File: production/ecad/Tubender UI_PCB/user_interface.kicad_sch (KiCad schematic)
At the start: 20 parts, among them IC3 SN74LVC1G29DCTR, J1 640387-5, J2 1-640387-0, J3 104031-0811, J4 640387-5, J5 4-1734592-0, J6 4-1734592-0, U5 74HC595, U6 PEC11R-4215K-S0024

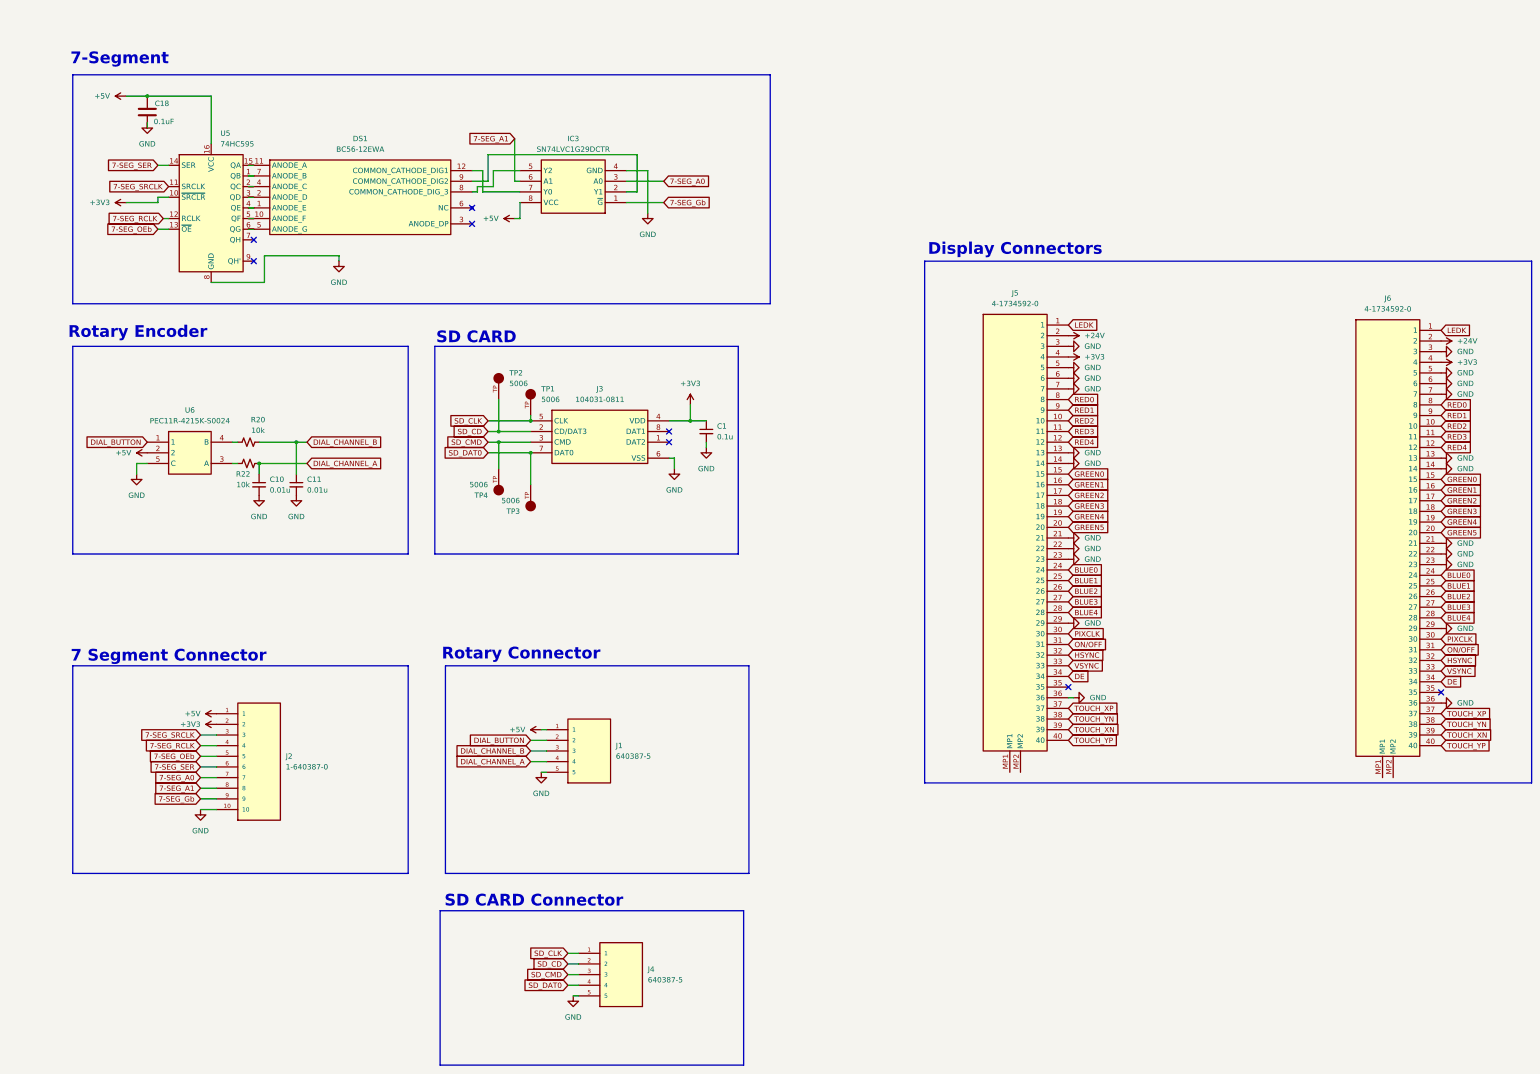
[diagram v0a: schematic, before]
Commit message: Finished First Draft Layout of UI PCB
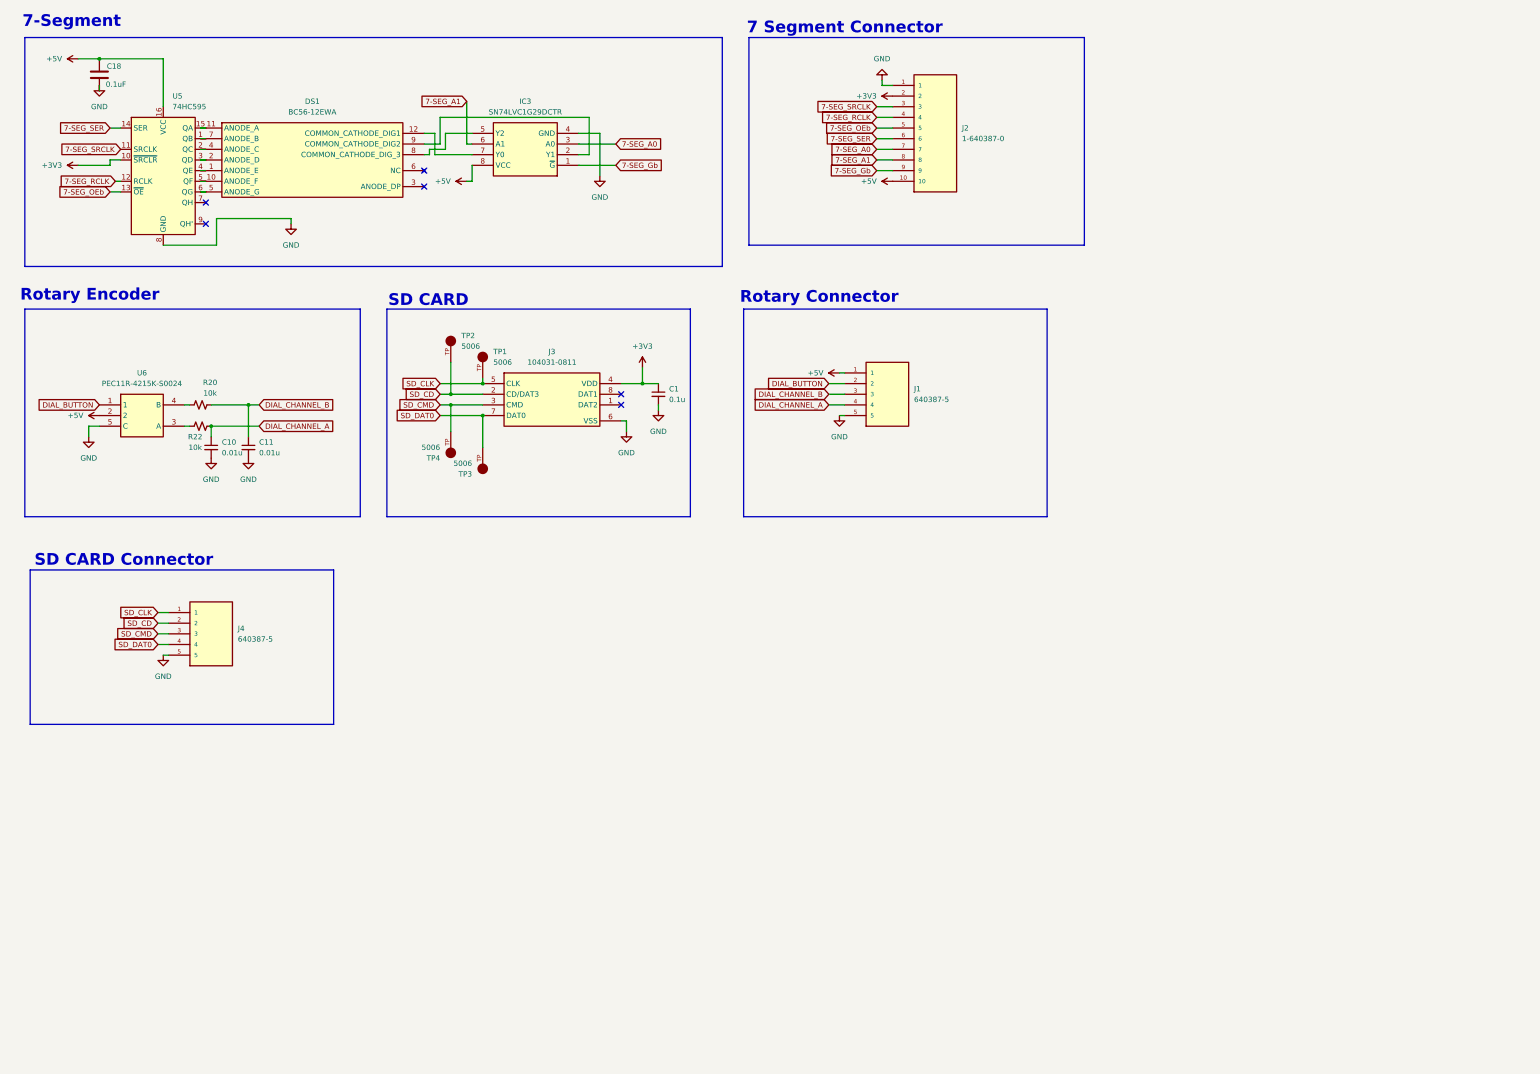
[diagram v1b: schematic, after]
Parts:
- removed J5, J6: 4-1734592-0, footprints:TE_4-1734592-0, symbol SamacSys_Parts:4-1734592-0
- IC3: footprint footprints:DCT0008A_N -> footprints:SOP65P400X130-8N
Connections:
- net +5V: now also J2.10; no longer J2.1
- net GND: now also J2.1; no longer J2.10
- no-connect marks 8 -> 6
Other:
- note removed: "Display Connectors"
- moved on the sheet: C1, C10, C11, C18, DS1, IC3, J1, J2, J3, J4, R20, R22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
